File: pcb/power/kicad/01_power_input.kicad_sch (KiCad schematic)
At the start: 31 parts, among them CN1 XT60PW-M / 三串电池, Q1 IRF4905, Q3 IRF4905, Q4 MMBT3904, U21 TL431BIDBZR, U22 LM393BIDR, U23 LM393BIDR

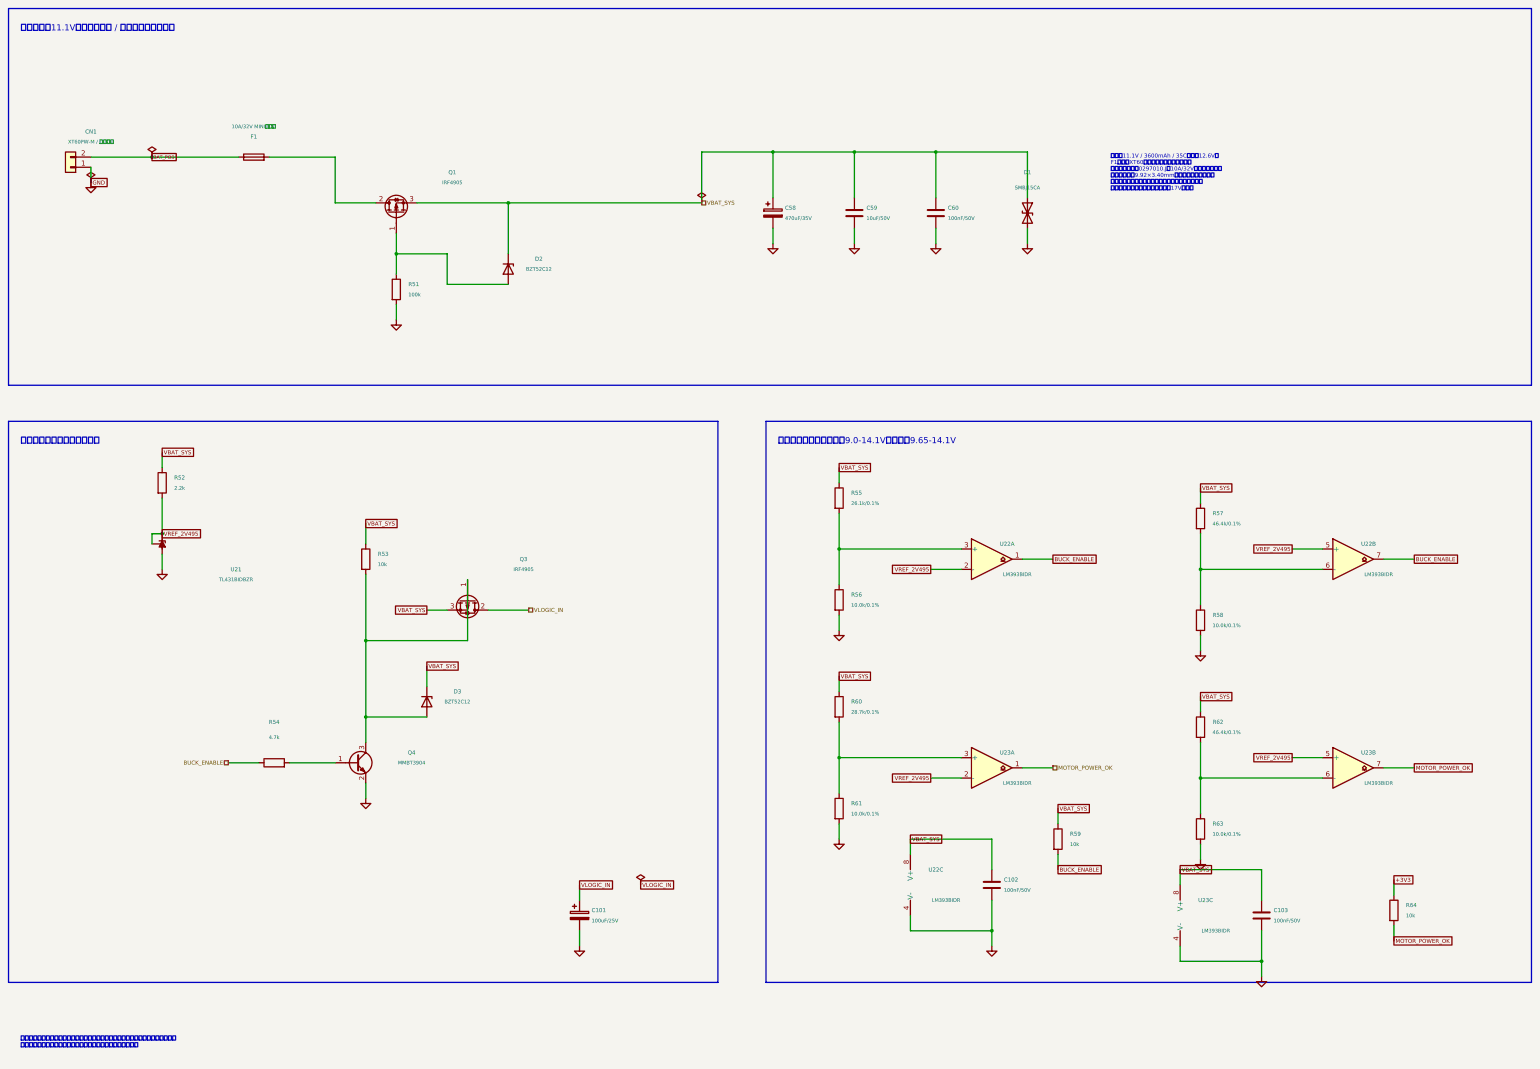
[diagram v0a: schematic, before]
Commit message: 10.4
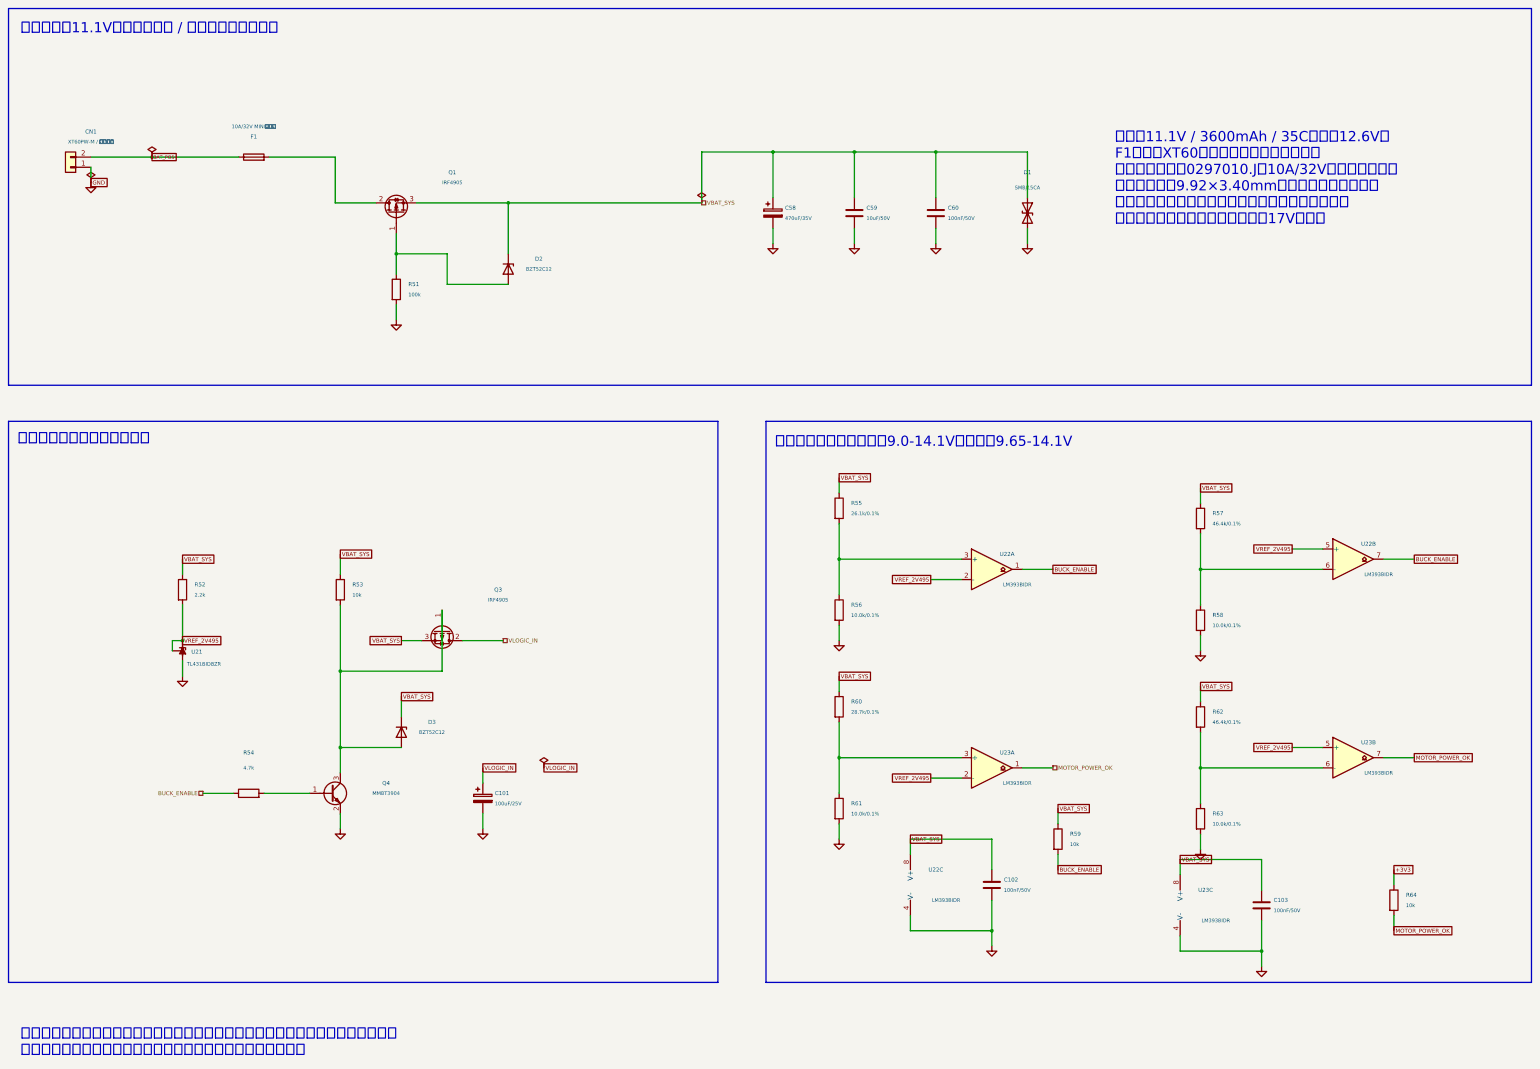
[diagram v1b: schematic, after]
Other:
- moved on the sheet: C101, C103, D3, Q3, Q4, R52, R53, R54, R55, R56, R62, R63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
